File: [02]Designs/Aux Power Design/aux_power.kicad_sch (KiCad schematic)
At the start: 26 parts, among them T1 Transformer_1P_2S, T2 Transformer_1P_2S, U1 LM7815_TO220, U2 LM7812_TO220, U3 LM7812_TO220, U4 LM78L05_SO8, U5 LD1117S33TR_SOT223, U6 LM7815_TO220, U7 LM7815_TO220, U8 LM7815_TO220, U9 LM7815_TO220

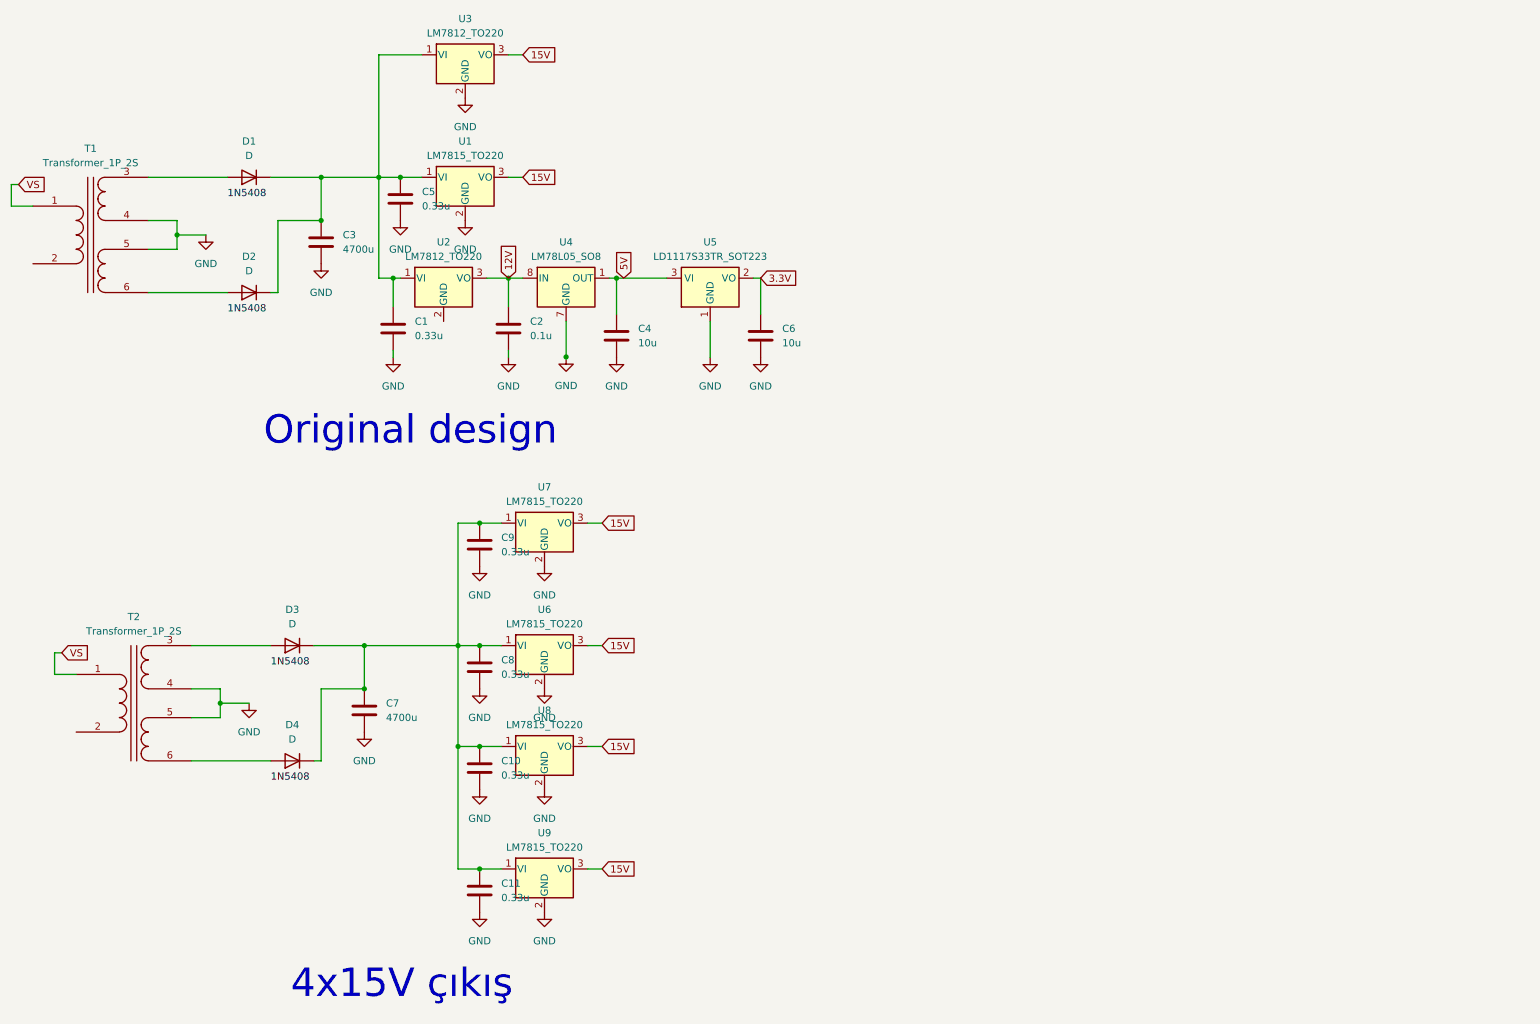
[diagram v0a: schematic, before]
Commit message: Schematic and Footprints are finished
Co-Authored-By: KaanDemirkoparan <57269134+KaanDemirkoparan@users.noreply.github.com>
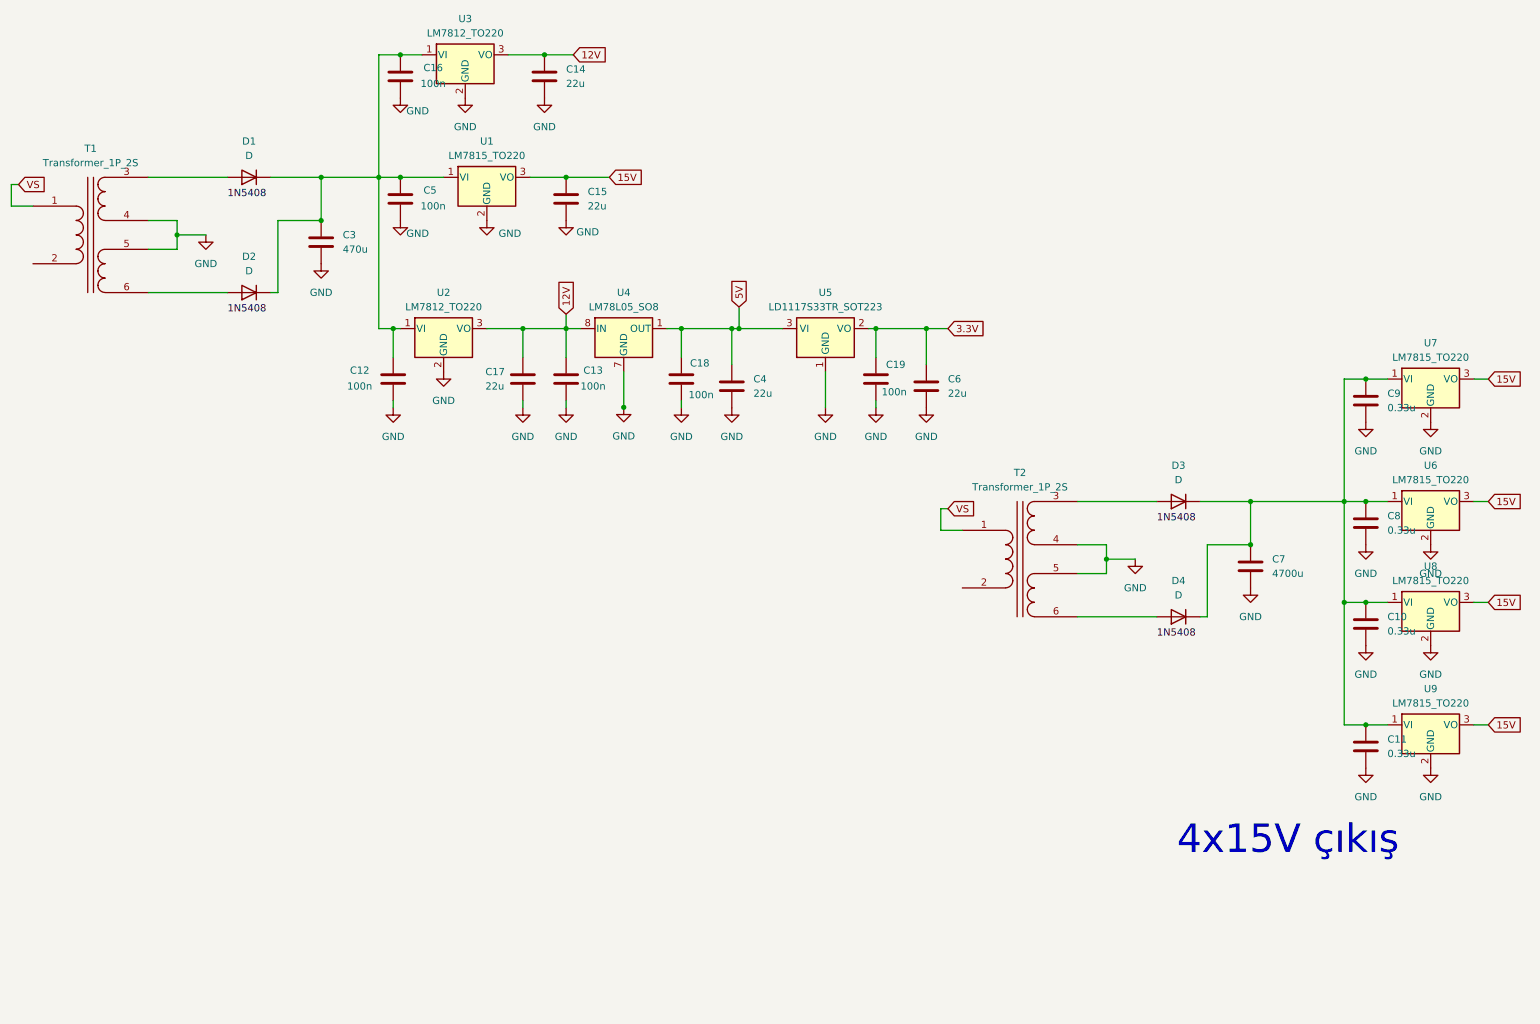
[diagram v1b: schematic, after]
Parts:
- removed C1: 0.33u, symbol Device:C
- removed C2: 0.1u, symbol Device:C
- added C12, C13, C16, C18, C19: 100n, symbol Device:C
- added C14, C15, C17: 22u, symbol Device:C
- C3: value 4700u -> 470u
- C4, C6: value 10u -> 22u
- C5: value 0.33u -> 100n
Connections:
- net 12V: now also U3.3 (VO), C13.1, C14.1, C17.1
- net 15V: now also C15.1; no longer U3.3 (VO)
- net 3.3V: now also C19.1
- net 5V: now also C18.1
- net GND: now also U2.2 (GND), C12.2, C13.2, C14.2, C15.2, C16.2, C17.2, C18.2, C19.2
- net at C3.1, C5.1, D1.1 (K)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: now also C12.1, C16.1
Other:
- note removed: "Original design"
- moved on the sheet: C10, C11, C4, C7, C8, C9, D3, D4, T2, U1, U2, U4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
